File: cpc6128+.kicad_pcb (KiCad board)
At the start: 2 copper layers, 284 x 140.5 mm, 199 parts, among them IC101 AMS40489, IC102 z80_6128, IC103 SED9420Cac, IC104 UPD765AC-2, IC105 74LS38, IC106 74LS38, IC107 74HC14, IC108 MC74HC4051N, IC109 LA6393D, IC110 41464, IC111 41464, IC112 41464, IC113 41464, IC114 AY38912, IC115 AMS40464, IC116 74HCT02, J101 rj12, J102 audio/video, J103 Jack audio, J104 POWER_JACK_6128, Q101 KTC1815Y, Q103 KTC1815Y, Q104 KTC1815Y, Q105 KTC1815Y, Q106 KTC1815Y, Q107 KTC1815Y, SW1 SW_DIP_x01, X181 40 MHz

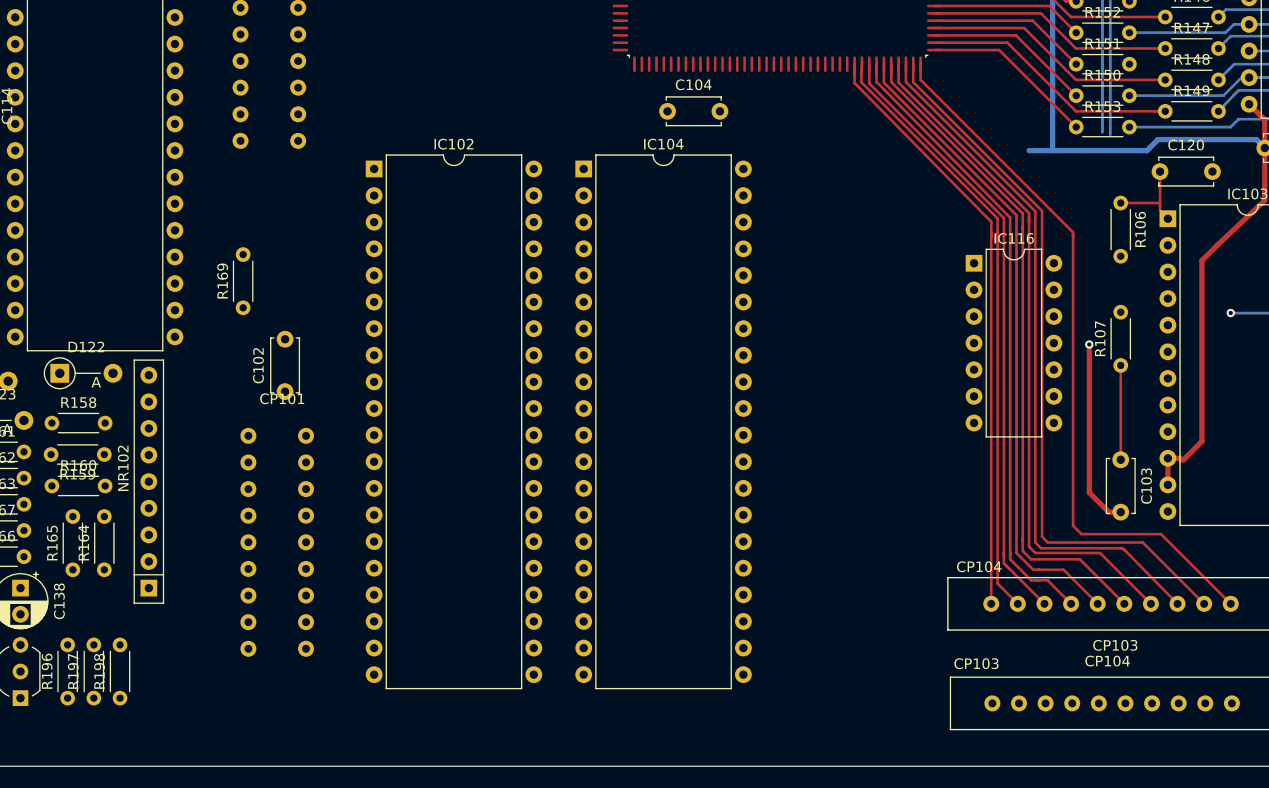
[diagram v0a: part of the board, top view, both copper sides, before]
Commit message: Cabled the keyboard
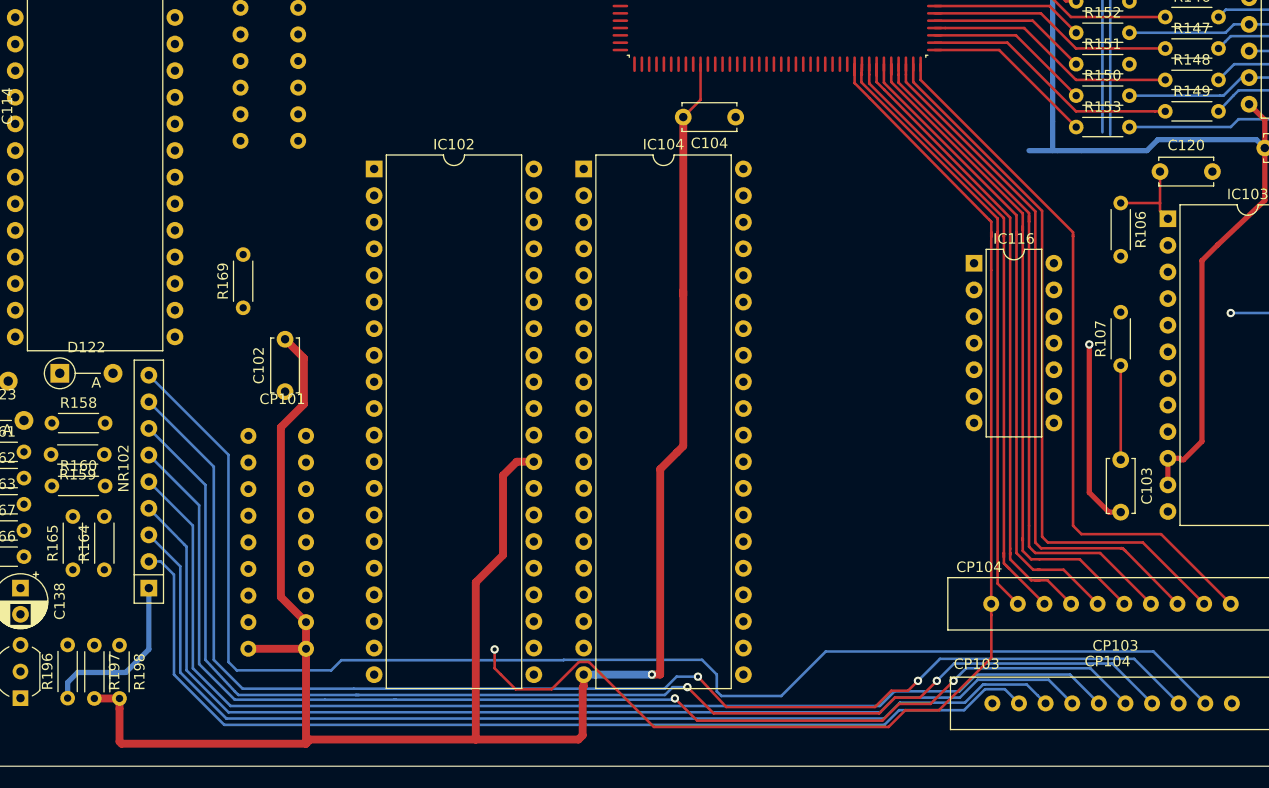
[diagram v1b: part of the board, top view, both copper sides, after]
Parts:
- moved C104 6.52 mm to (120.5, 100.8), turned to 180 degrees
- moved R197 5.05 mm to (59.3, 151.2), turned to 270 degrees
- moved R198 5.05 mm to (61.7, 151.2), turned to 270 degrees
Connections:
- NR102 pad 2: Net-(NR102-Pad2) -> X8
- NR102 pad 3: Net-(NR102-Pad3) -> X7
- NR102 pad 4: Net-(NR102-Pad4) -> X6
- NR102 pad 5: Net-(NR102-Pad5) -> X5
- NR102 pad 6: Net-(NR102-Pad6) -> X4
- NR102 pad 7: Net-(NR102-Pad7) -> X3
- NR102 pad 8: Net-(NR102-Pad8) -> X2
- NR102 pad 9: Net-(NR102-Pad9) -> X1
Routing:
- net GND: track 704.7 -> 906.1 mm, vias 2 -> 3
- net X1: track 0.00 -> 130.7 mm
- net X2: track 0.00 -> 125.8 mm, vias 0 -> 2
- net X3: track 0.00 -> 121.3 mm, vias 0 -> 2
- net X4: track 0.00 -> 116.4 mm, vias 0 -> 2
- net X5: track 0.00 -> 109.9 mm
- net X6: track 0.00 -> 105.3 mm
- net X7: track 0.00 -> 101.1 mm
- net X8: track 0.00 -> 97.0 mm
- net Y10: track 58.3 -> 119.8 mm, vias 0 -> 1
- net +5V: track 485.6 -> 502.0 mm
